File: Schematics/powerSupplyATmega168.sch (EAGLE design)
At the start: 5 parts, among them IC1 LM2931T

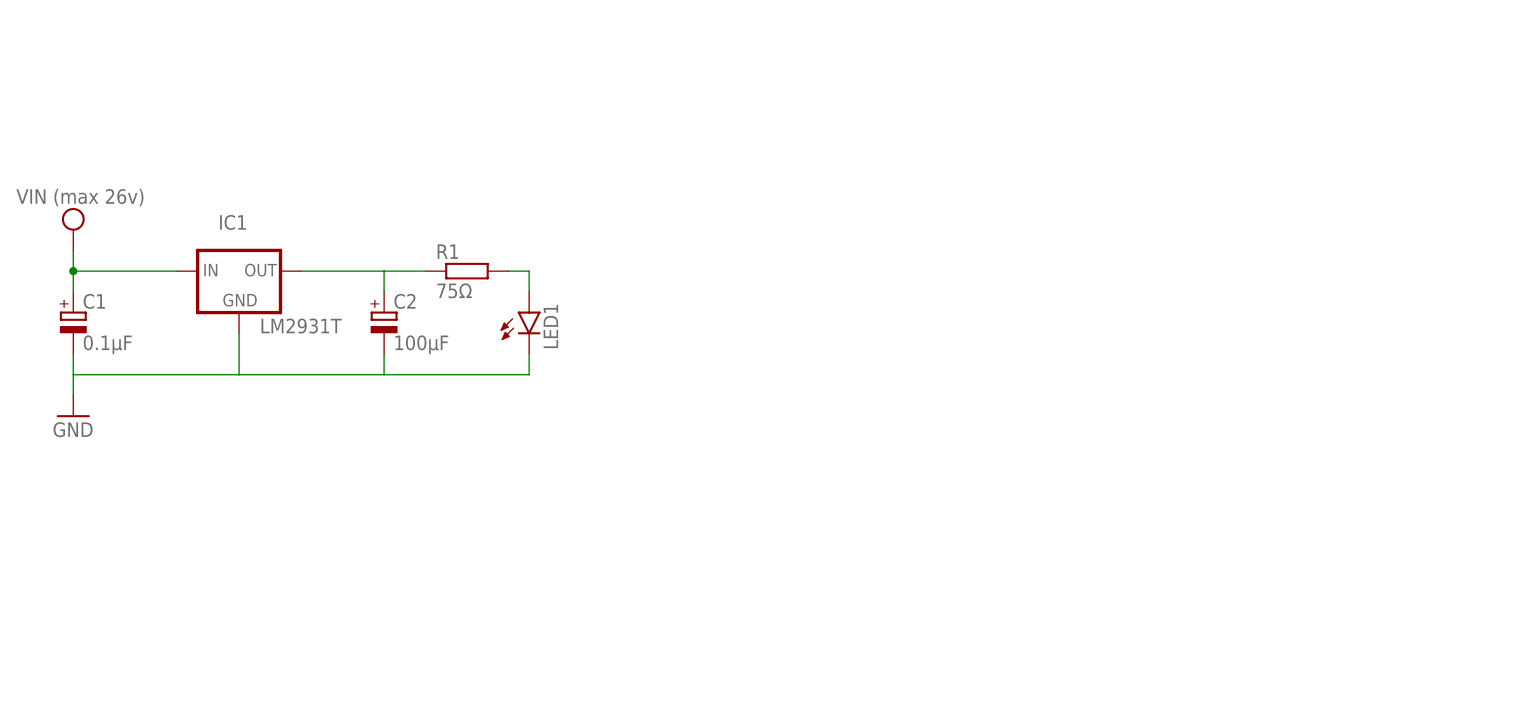
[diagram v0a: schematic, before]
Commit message: Added different schematics and code
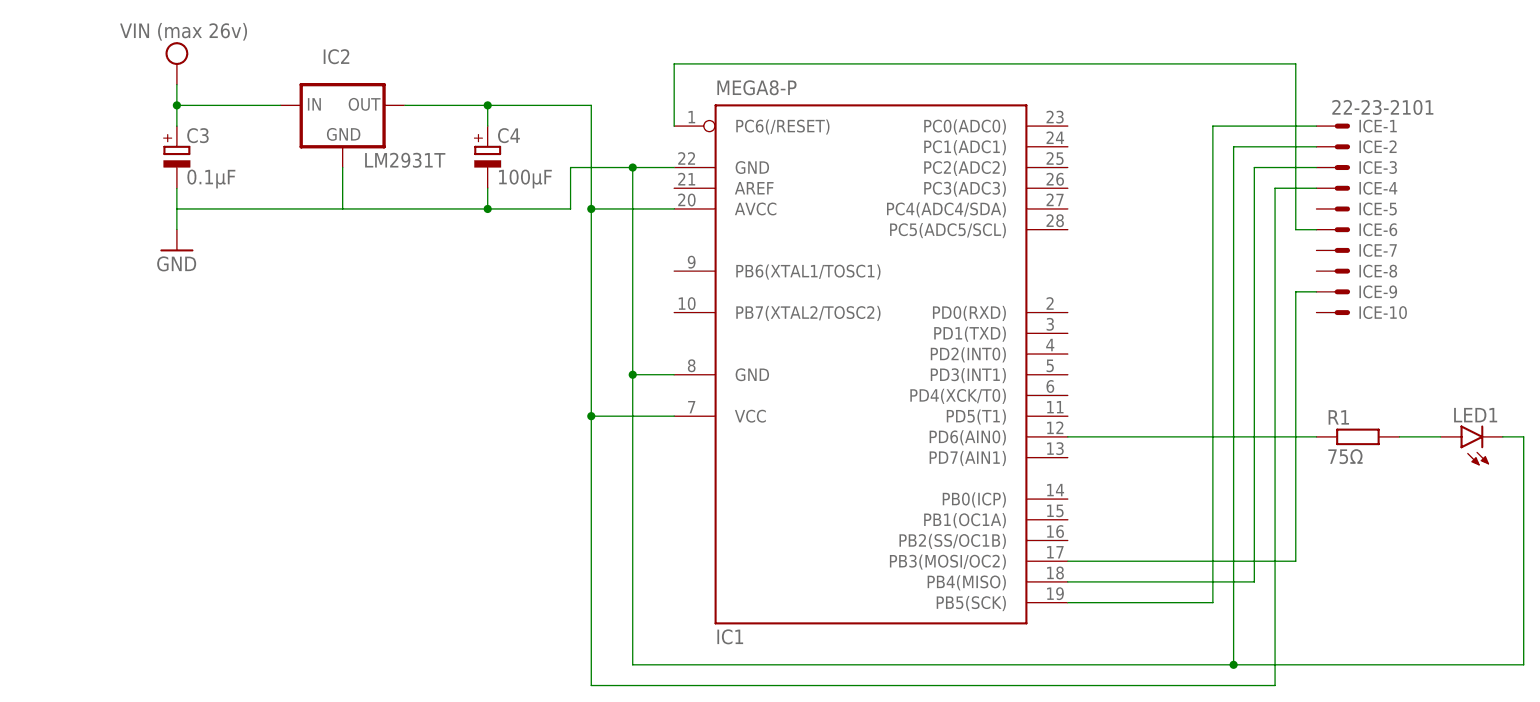
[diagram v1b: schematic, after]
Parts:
- removed C1: 0.1µF, rcl:CPOL-EUE5-5
- removed C2: 100µF, rcl:CPOL-EUE5-5
- added C3: 0.1µF, rcl:CPOL-EUE5-5
- added C4: 100µF, rcl:CPOL-EUE5-5
- added IC2: LM2931T, v-reg-3:LM2931T
- added ICE: 22-23-2101, con-molex:22-23-2101
- IC1: value LM2931T -> MEGA8-P; device v-reg-3:LM2931T -> atmel:MEGA8-P
- LED1: value (none) -> SFH482; device led:LED5MM -> led:SFH482
- R1: device rcl:R-EU_0204/7 -> rcl:R-EU_0617/17
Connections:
- removed net N$1 (its old number): C2.+, IC1.OUT, R1.1
- new net N$2: IC1.PB5(SCK), ICE-1.S
- new net N$4: C4.+, IC1.AVCC, IC1.VCC@1, IC2.OUT, ICE-4.S
- new net N$5: IC1.PC6(/RESET), ICE-6.S
- new net N$6: IC1.PB3(MOSI/OC2), ICE-9.S
- new net N$7: IC1.PD6(AIN0), R1.1
- net GND: now also C3.-, C4.-, IC1.GND@1, IC2.GND, ICE-2.S; no longer C1.-
- net N$3: now also IC1.PB4(MISO), ICE-3.S; no longer C2.-
- net VCC: now also C3.+, IC2.IN; no longer C1.+, IC1.IN
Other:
- moved on the sheet: R1
